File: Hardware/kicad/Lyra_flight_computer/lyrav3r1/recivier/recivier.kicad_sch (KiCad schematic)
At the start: 88 parts, among them J1 USB_B_Micro, J2 Conn_01x02, J3 Conn_01x02, J4 Screw_Terminal_01x02, J5 Screw_Terminal_01x02, Q1 AO3401A, SW1 K2-1102DP-L3SW-04, SW2 K2-1102DP-L3SW-04, SW3 K2-1102DP-L3SW-04, SW4 K2-1102DP-L3SW-04, SW5 K2-1102DP-L3SW-04, SW6 SW_SPDT, U1 E22-900MM22S, U2 W25Q128JVS, U3 RP2040, U4 TXB0104RGY, U5 PCM5102A, U6 ATGM336H-5N31, U7 LIS3MDLTR, U8 AMS1117-3.3, U9 AMS1117-5.0, X1 SX1M12.000M10F30TNN

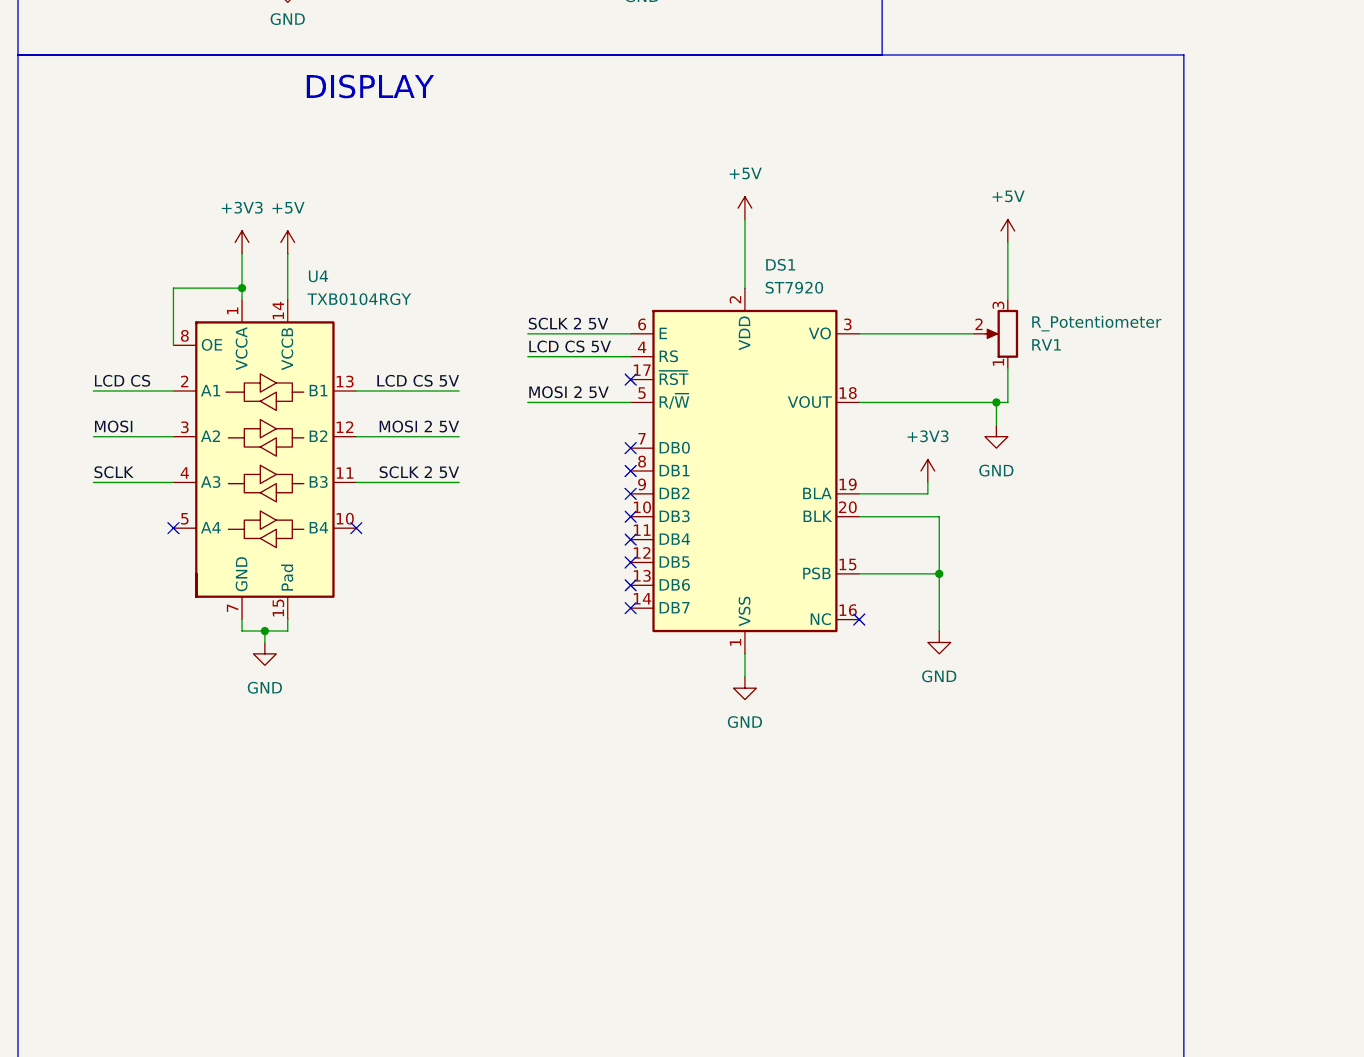
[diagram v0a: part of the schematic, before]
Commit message: reciver rework
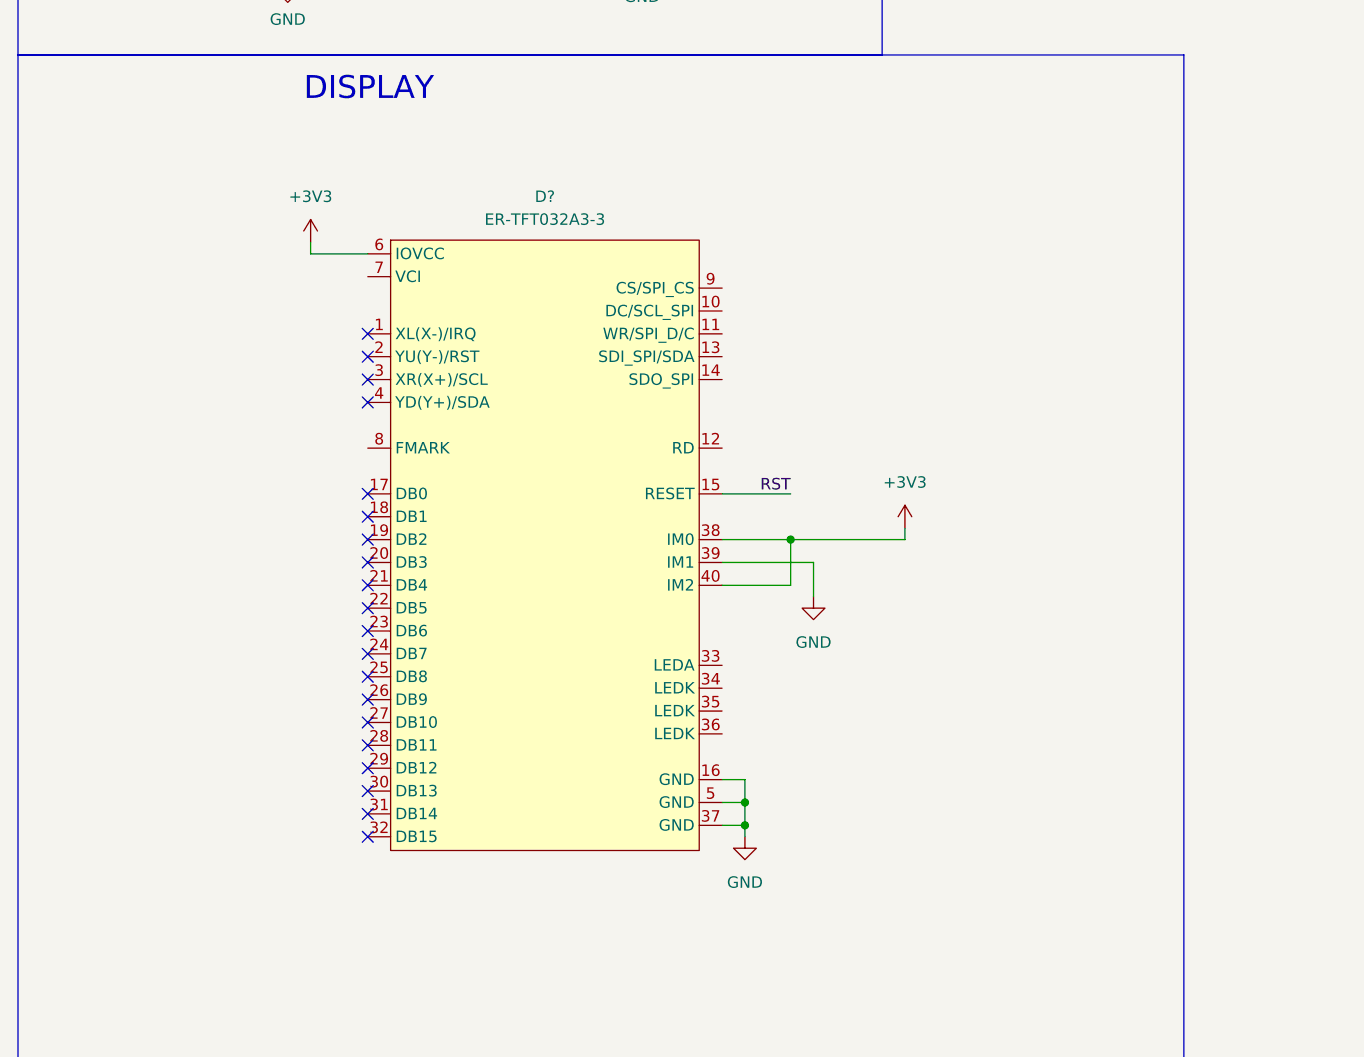
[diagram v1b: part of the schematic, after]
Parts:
- removed DS1: ST7920, .pretty:ST7920 AZ, symbol Display_Graphic:ERM19264
- removed RV1: R_Potentiometer, .pretty:RES-ADJ-SMD_3314J, symbol Device:R_Potentiometer
- removed U4: TXB0104RGY, Package_DFN_QFN:Texas_S-PVQFN-N14, symbol Logic_LevelTranslator:TXB0104RGY
- added D?: ER-TFT032A3-3, .pretty:FPC-SMD_40P-P0.50_AMPHENOL_62684-402100ALF, symbol .kicad_sym:ER-TFT032IPS_LCD
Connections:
- net +3.3VA: now also D?.38 (IM0), D?.40 (IM2), D?.6 (IOVCC)
- net GND: now also D?.16 (GND), D?.37 (GND), D?.39 (IM1), D?.5 (GND)
- new net RST: D?.15 (RESET)
- no-connect marks 59 -> 67
